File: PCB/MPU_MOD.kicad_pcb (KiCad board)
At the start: 8 copper layers, 43.5 x 70 mm, 266 parts, among them J1 SJ-43504-SMT-TR, J2 2-1734248-0, J3 USB4510-03-1-A_REVA, J501 MEM2090-00-145-00-A_REVA, J701 FTSH-107-01-L-DV-K-A, J901 73412-0110, U1 IS21ES08GA-JQLI-TR, U201 STC3115IQT, U203 STPMIC1APQR, U3 BQ24298RTWR, U301 STM32MP157FABx, U401 MT41K256M16TW-107_P, U502 HSP051-4M10, U503 HSP051-4M10, U701 HSP051-4M10, U702 HSP051-4M10, U801 FUSB302BMPX, U802 HSP051-4M10, U901 LBEE5PK2AE-771, Y601 NX2012SA-32.768K, Y701 ECS-2520MVQ-240

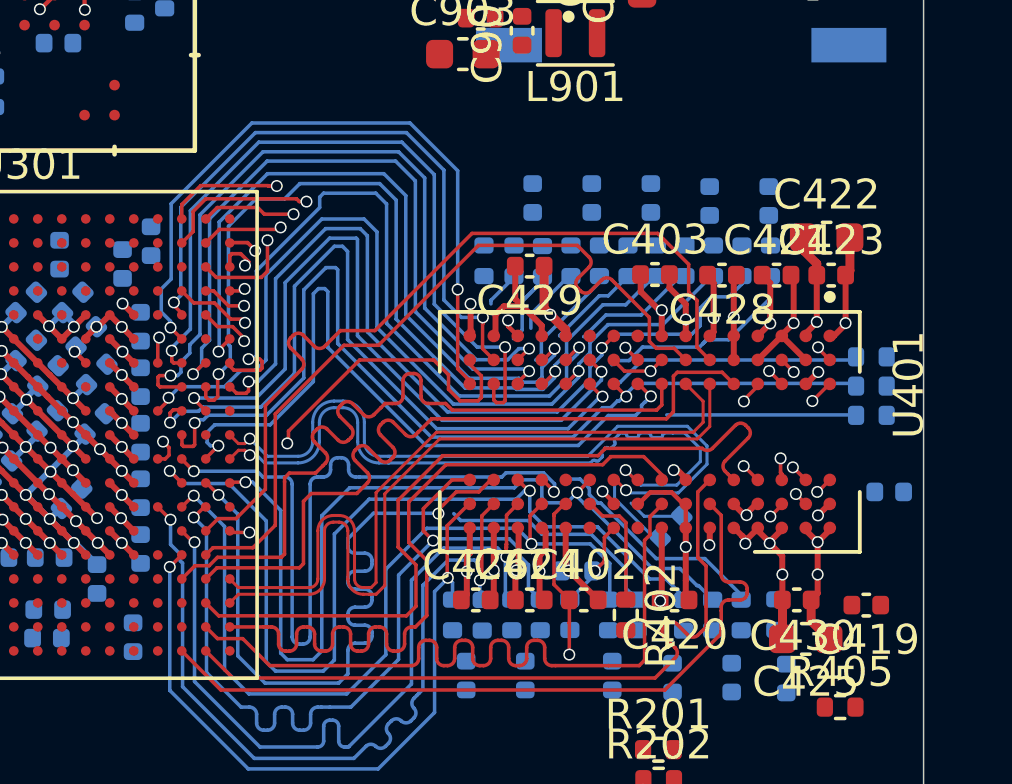
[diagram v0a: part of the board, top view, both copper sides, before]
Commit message: PCB_update
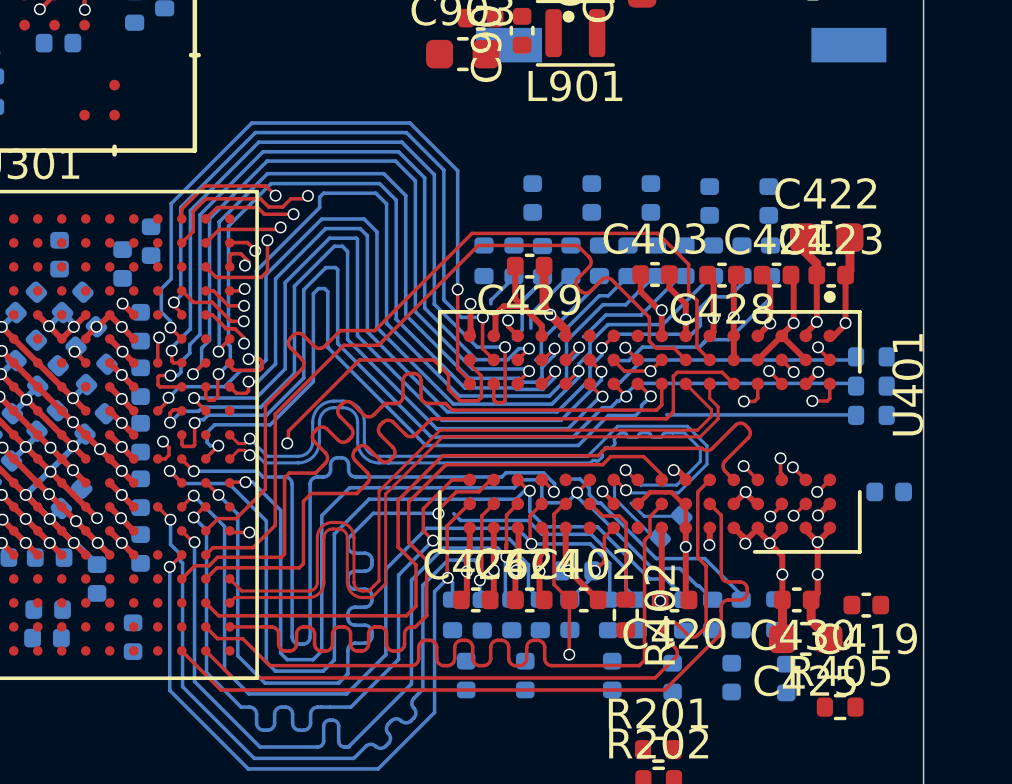
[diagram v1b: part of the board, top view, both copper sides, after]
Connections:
- U401 pad A2: /DDR/DDR_DQ0 -> /DDR/DDR_DQ3
- U401 pad B8: /DDR/DDR_DQ5 -> /DDR/DDR_DQ4
- U401 pad C2: /DDR/DDR_DQ3 -> /DDR/DDR_DQ0
- U401 pad C8: /DDR/DDR_DQ4 -> /DDR/DDR_DQ5
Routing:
- net /DDR/DDR_DQM0: track 22.4 -> 25.1 mm
- net /DDR/DDR_DQ1: track 22.2 -> 23.8 mm
- net /DDR/DDR_DQ5: track 25.2 -> 24.1 mm
- net /DDR/DDR_DQ0: track 25.3 -> 24.2 mm
- net /DDR/DDR_DQ7: track 23.7 -> 24.6 mm
- net /DDR/DDR_DQ3: track 24.4 -> 25.3 mm
- net /DDR/DDR_A0: track 29.4 -> 28.7 mm
